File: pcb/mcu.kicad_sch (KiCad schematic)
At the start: 30 parts, among them J1 RC555, J2 pa1010d, J4 USB_C_Receptacle_USB2.0_16P, J5 UART, Q1 AO3401A, Q2 SS8050, Q3 SS8050, SW2 SW_Push, SW3 SW_Push, U3 ESP32-S3-WROOM-1

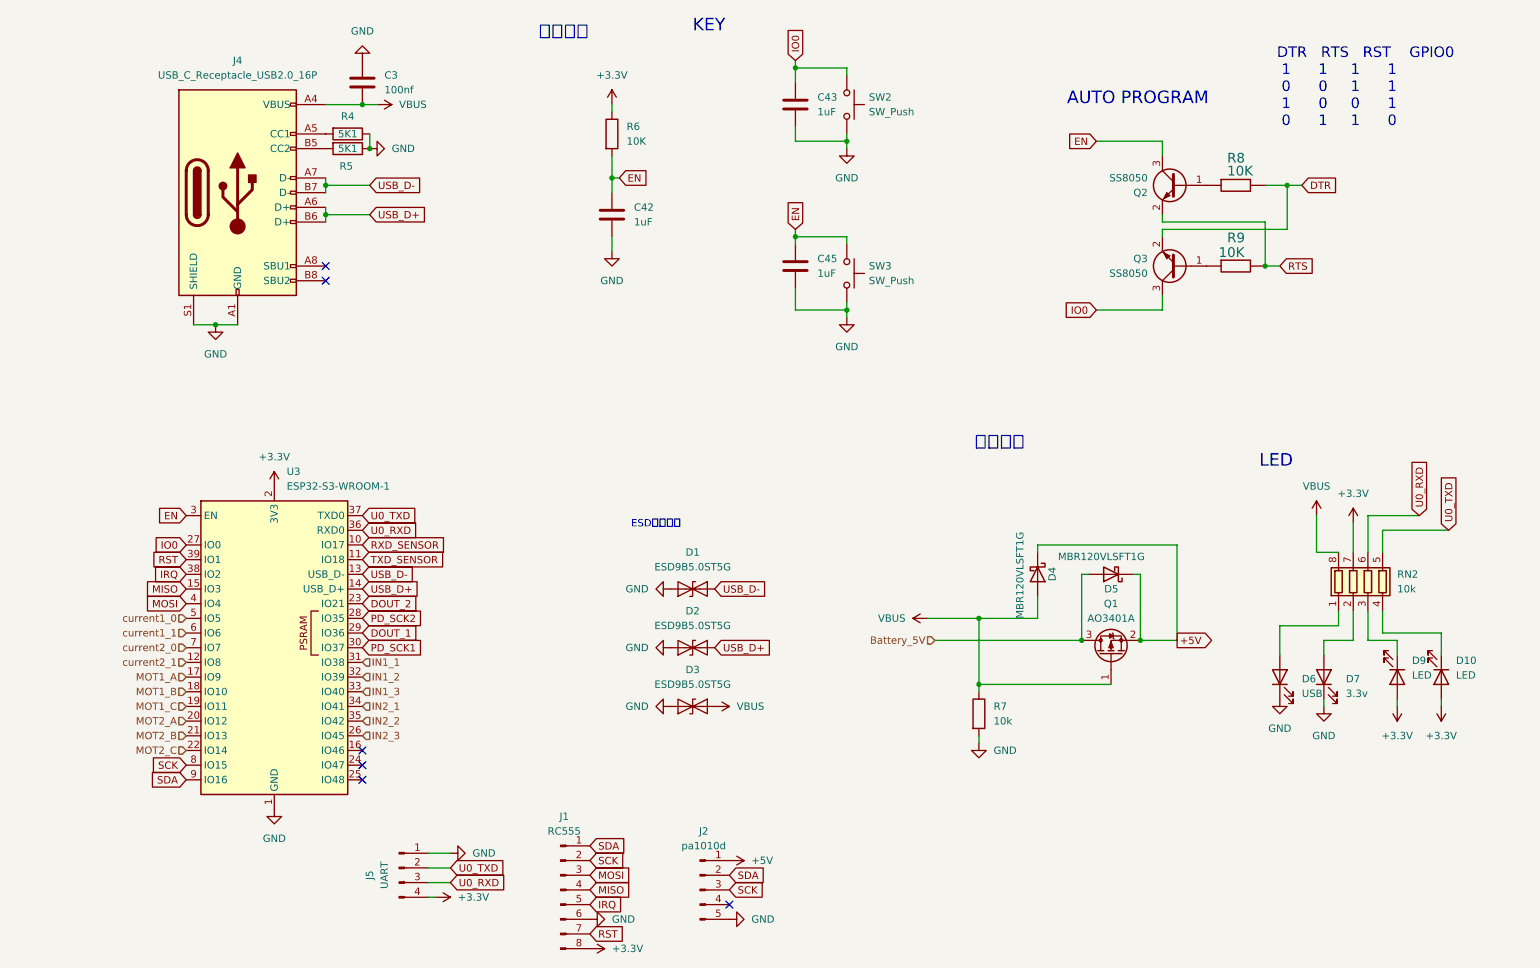
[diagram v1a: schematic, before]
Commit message: feat: update
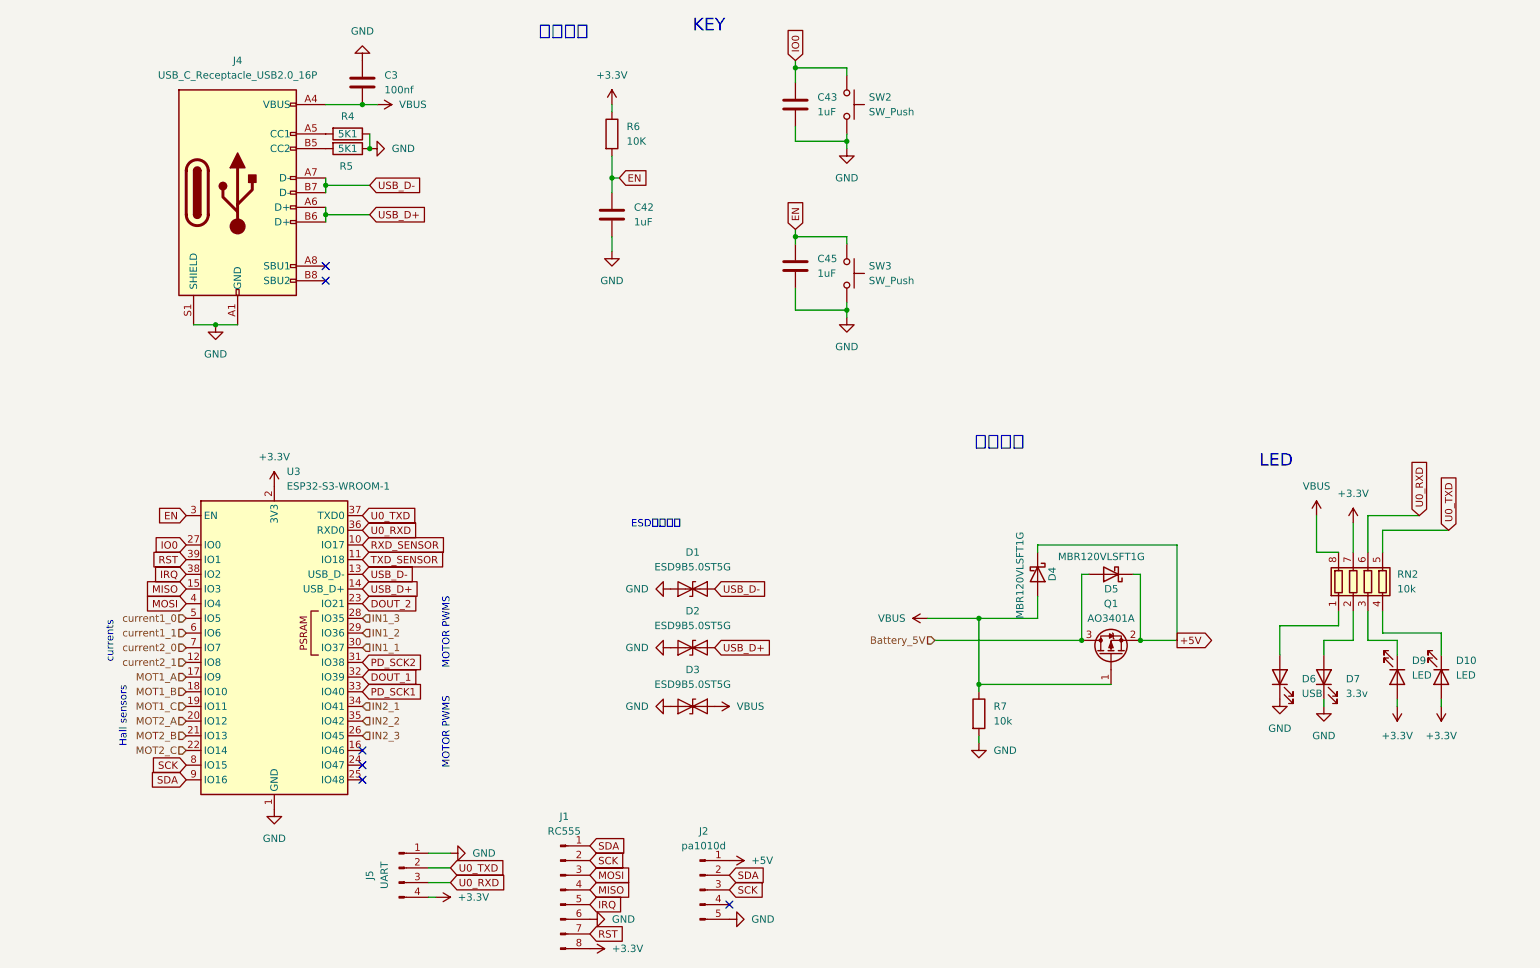
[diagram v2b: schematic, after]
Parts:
- removed Q2, Q3: SS8050, Package_TO_SOT_SMD:SOT-23, symbol Transistor_BJT:SS8050
- removed R8: 10K, Resistor_SMD:R_0603_1608Metric, symbol CR0402JF0101G_2
- removed R9: 10K, Resistor_SMD:R_0603_1608Metric, symbol CR0402JF0101G_3
- J1: footprint Connector_PinHeader_2.54mm:PinHeader_1x08_P2.54mm_Vertical -> Connector_JST:JST_PH_B8B-PH-K_1x08_P2.00mm_Vertical
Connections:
- net DOUT_1: now also U3.32 (IO39); no longer U3.29 (IO36)
- net IN1_1: now also U3.30 (IO37); no longer U3.31 (IO38)
- net IN1_2: now also U3.29 (IO36); no longer U3.32 (IO39)
- net IN1_3: now also U3.28 (IO35); no longer U3.33 (IO40)
- net PD_SCK1: now also U3.33 (IO40); no longer U3.30 (IO37)
- net PD_SCK2: now also U3.31 (IO38); no longer U3.28 (IO35)
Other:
- note added: "Hall sensors"
- note added: "MOTOR PWMS"
- note added: "currents"
- note removed: "AUTO PROGRAM"
- note removed: "DTR RTS RST GPIO0 1 1 1 1 0 0 1 1 1 0 0 1 0 1 1 0"

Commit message: feat: update
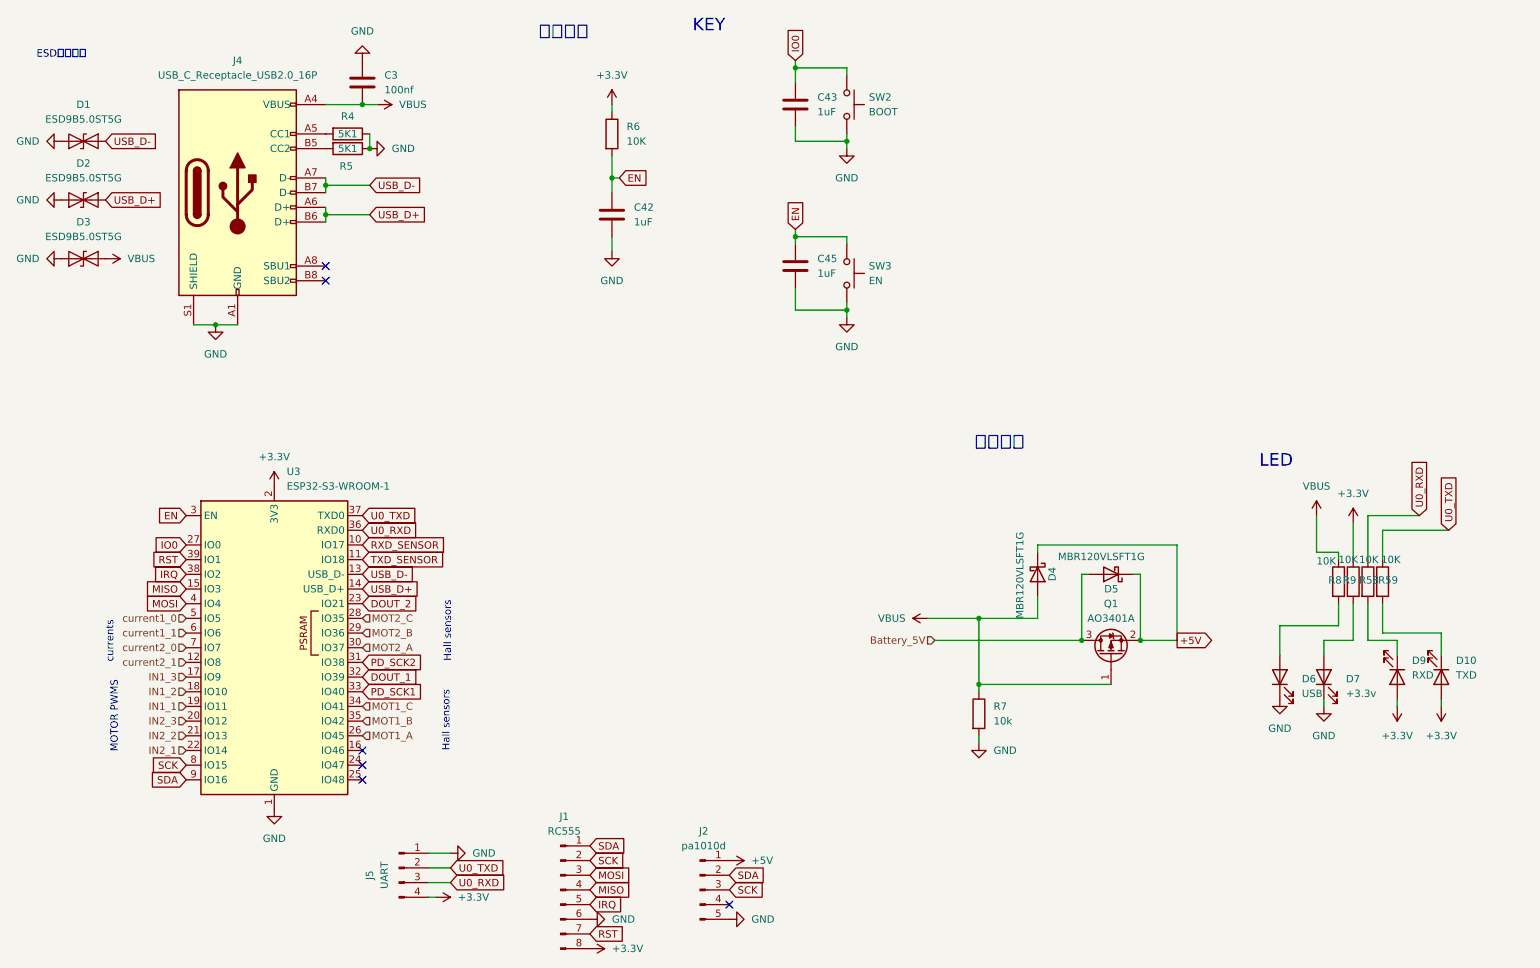
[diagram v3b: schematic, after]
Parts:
- removed RN2: 10k, Resistor_SMD:R_Array_Concave_4x0603, symbol Device:R_Pack04
- added R58, R59, R8, R9: 10K, Resistor_SMD:R_0603_1608Metric, symbol Device:R
- D10: value LED -> TXD
- D7: value 3.3v -> +3.3v
- D9: value LED -> RXD
- SW2: value SW_Push -> BOOT
- SW3: value SW_Push -> EN
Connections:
- net +3.3V: now also R9.1
- net IN1_1: now also U3.19 (IO11); no longer U3.30 (IO37)
- net IN1_2: now also U3.18 (IO10); no longer U3.29 (IO36)
- net IN1_3: now also U3.17 (IO9); no longer U3.28 (IO35)
- net IN2_1: now also U3.22 (IO14); no longer U3.34 (IO41)
- net IN2_2: now also U3.21 (IO13); no longer U3.35 (IO42)
- net IN2_3: now also U3.20 (IO12); no longer U3.26 (IO45)
- net MOT1_A: now also U3.26 (IO45); no longer U3.17 (IO9)
- net MOT1_B: now also U3.35 (IO42); no longer U3.18 (IO10)
- net MOT1_C: now also U3.34 (IO41); no longer U3.19 (IO11)
- net MOT2_A: now also U3.30 (IO37); no longer U3.20 (IO12)
- net MOT2_B: now also U3.29 (IO36); no longer U3.21 (IO13)
- net MOT2_C: now also U3.28 (IO35); no longer U3.22 (IO14)
- net U0_RXD: now also R58.1
- net U0_TXD: now also R59.1
- net VBUS: now also R8.1
- net at D6.2 (A): now also R8.2
- net at D7.2 (A): now also R9.2
- net at D9.1 (K): now also R58.2
- net at D10.1 (K): now also R59.2
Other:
- moved on the sheet: D1, D2, D3

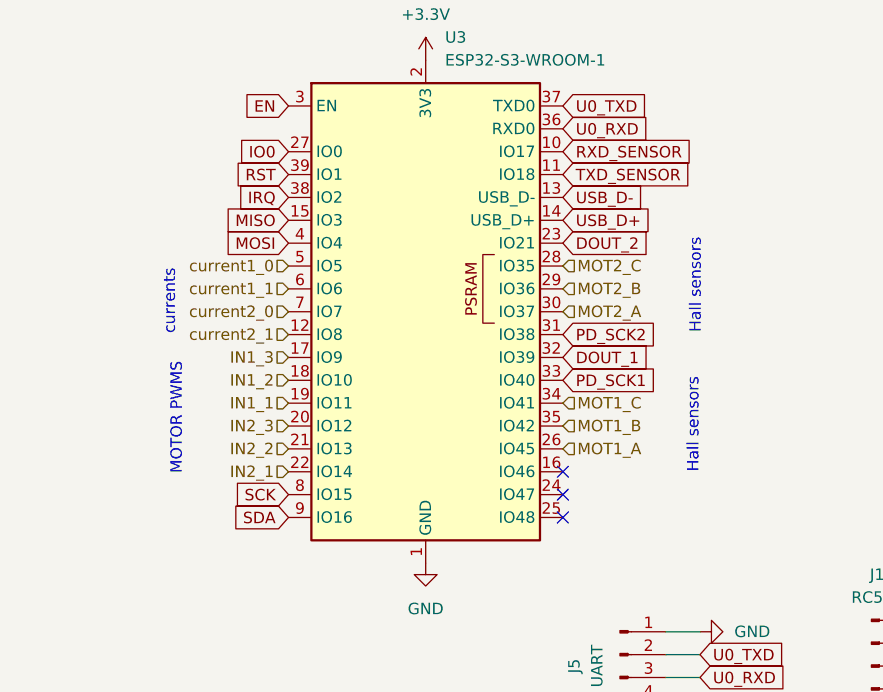
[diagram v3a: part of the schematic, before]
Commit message: feat: update
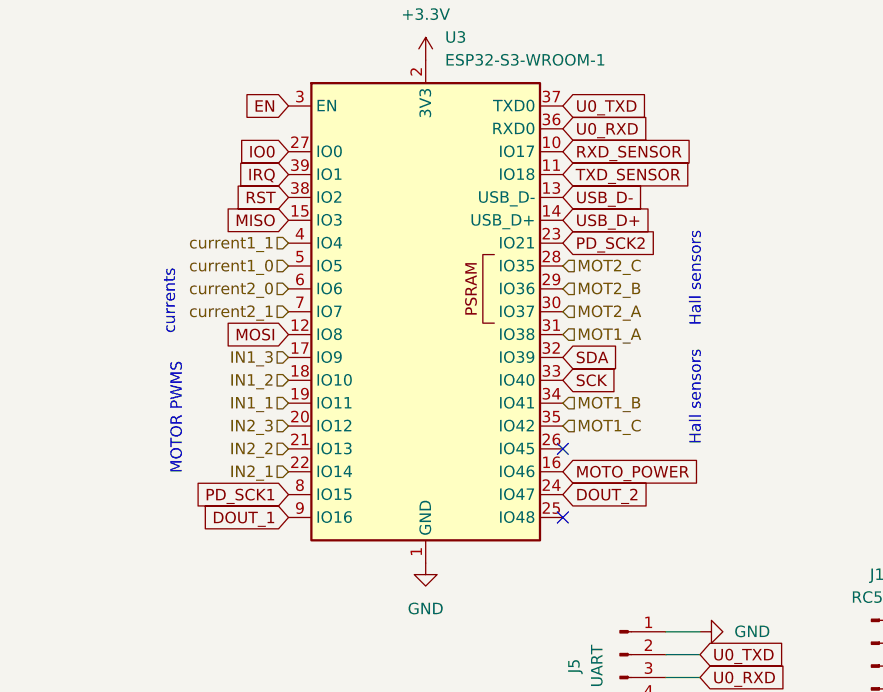
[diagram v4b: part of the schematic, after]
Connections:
- net DOUT_1: now also U3.9 (IO16); no longer U3.32 (IO39)
- net DOUT_2: now also U3.24 (IO47); no longer U3.23 (IO21)
- net IRQ: now also U3.39 (IO1); no longer U3.38 (IO2)
- net MOSI: now also U3.12 (IO8); no longer U3.4 (IO4)
- net MOT1_A: now also U3.31 (IO38); no longer U3.26 (IO45)
- net MOT1_B: now also U3.34 (IO41); no longer U3.35 (IO42)
- net MOT1_C: now also U3.35 (IO42); no longer U3.34 (IO41)
- net PD_SCK1: now also U3.8 (IO15); no longer U3.33 (IO40)
- net PD_SCK2: now also U3.23 (IO21); no longer U3.31 (IO38)
- net RST: now also U3.38 (IO2); no longer U3.39 (IO1)
- net SCK: now also U3.33 (IO40); no longer U3.8 (IO15)
- net SDA: now also U3.32 (IO39); no longer U3.9 (IO16)
- net current1_1: now also U3.4 (IO4); no longer U3.6 (IO6)
- net current2_0: now also U3.6 (IO6); no longer U3.7 (IO7)
- net current2_1: now also U3.7 (IO7); no longer U3.12 (IO8)
- net MOTO_POWER: now reaches U3.16 (IO46)
- no-connect marks 6 -> 5
